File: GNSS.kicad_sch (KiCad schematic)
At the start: 9 parts, among them U14 SAM-M10Q-00B

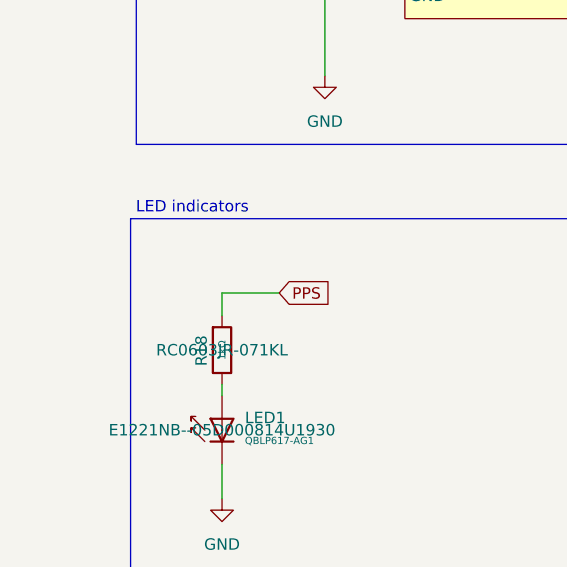
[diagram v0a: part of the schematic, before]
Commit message: Feat: Minor improvement
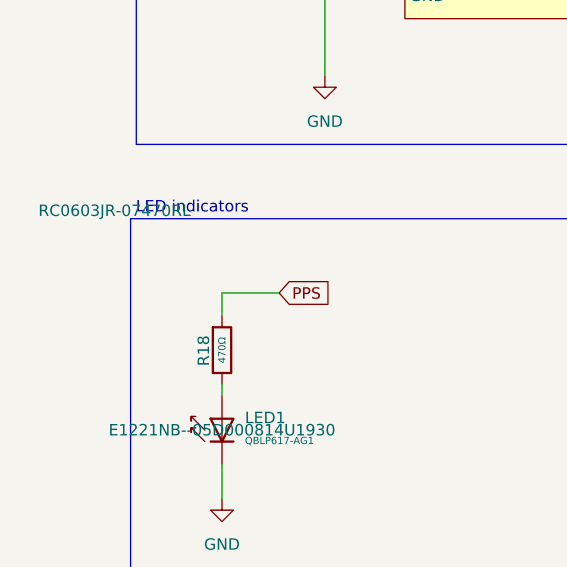
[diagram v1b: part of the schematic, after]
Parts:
- removed R18: 1kΩ, PCM_JLCPCB:R_0603, symbol PCM_JLCPCB-Resistors:0402,1kΩ
- added R18: 470Ω, PCM_JLCPCB:R_0603, symbol PCM_JLCPCB-Resistors:0402,470Ω
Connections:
- net PPS: now also R18.1
- net at LED1.2: now also R18.2
